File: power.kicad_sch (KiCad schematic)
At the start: 40 parts, among them SW7 Switch, U11 SY8079AAC, U12 SY8079AAC, U13 XT4054K421MR-G, U14 SY6280AAC, U15 SY6280AAC, U16 SY6280AAC

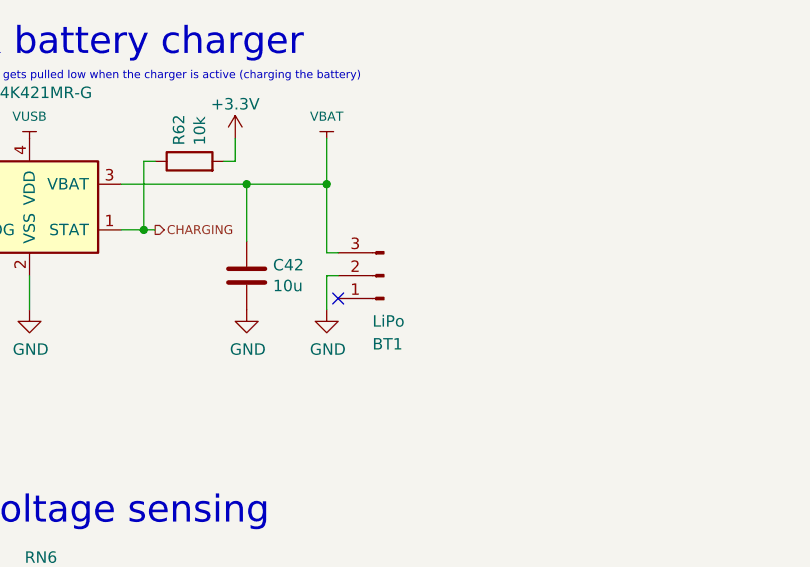
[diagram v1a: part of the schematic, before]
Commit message: Final version of prototype 4
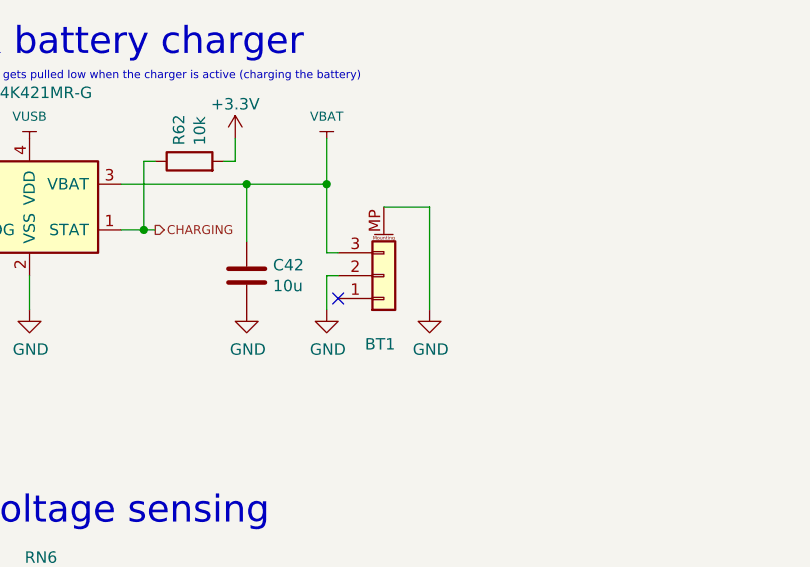
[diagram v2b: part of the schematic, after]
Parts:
- BT1: value LiPo -> (none); footprint Connector_JST:JST_PH_S3B-PH-SM4-TB_1x03-1MP_P2.00mm_Horizontal -> (none); symbol mch2021-rescue:Conn_01x03_Male-Connector -> Connector_Generic_MountingPin:Conn_01x03_MountingPin
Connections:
- net GND: now also BT1.MP (MountPin)
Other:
- moved on the sheet: BT1
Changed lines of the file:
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@@
+    (stroke (width 0) (type default) (color 0 0 0 0))
+  )
+  (wire (pts (xy 96.52 34.29) (xy 91.44 34.29))
     (stroke (width 0) (type default) (color 0 0 0 0))
   )
@@
   )
   (wire (pts (xy 58.42 85.09) (xy 64.77 85.09))
+    (stroke (width 0) (type default) (color 0 0 0 0))
+  )
+  (wire (pts (xy 96.52 45.72) (xy 96.52 34.29))
     (stroke (width 0) (type default) (color 0 0 0 0))
   )
@@
     (pin "1")
   )
-  (symbol (lib_id "mch2021-rescue:Conn_01x03_Male-Connector") (at 91.44 41.91 180) (unit 1)
-    (in_bom yes) (on_board yes)
-    (property "Reference" "BT1" (id 0) (at 90.17 49.53 0)
+  (symbol (lib_id "Connector_Generic_MountingPin:Conn_01x03_MountingPin") (at 91.44 41.91 0) (mirror x) (unit 1)
+    (in_bom yes) (on_board yes)
+    (property "Reference" "BT1" (id 0) (at 92.71 49.53 0)
       (effects (font (size 1.27 1.27)) (justify right))
     )
-    (property "Value" "LiPo" (id 1) (at 90.17 46.99 0)
+    (property "Value" "" (id 1) (at 92.71 46.99 0)
       (effects (font (size 1.27 1.27)) (justify right))
     )
-    (property "Footprint" "Connector_JST:JST_PH_S3B-PH-SM4-TB_1x03-1MP_P2.00mm_Horizontal" (id 2) (at 91.44 41.91 0)
+    (property "Footprint" "" (id 2) (at 91.44 41.91 0)
       (effects (font (size 1.27 1.27)) hide)
     )
@@
     (pin "2")
     (pin "3")
+    (pin "MP")
   )
   (symbol (lib_id "mch2021-rescue:AAT4610BIGV-1-T1-Power_Management") (at 156.21 109.22 0) (unit 1)
@@
     (pin "2")
   )
+  (symbol (lib_id "mch2021-rescue:GND-power") (at 96.52 45.72 0) (unit 1)
+    (in_bom yes) (on_board yes)
+    (property "Reference" "#PWR?" (id 0) (at 96.52 52.07 0)
+      (effects (font (size 1.27 1.27)) hide)
+    )
+    (property "Value" "GND" (id 1) (at 96.647 50.1142 0))
+    (property "Footprint" "" (id 2) (at 96.52 45.72 0)
+      (effects (font (size 1.27 1.27)) hide)
+    )
+    (property "Datasheet" "" (id 3) (at 96.52 45.72 0)
+      (effects (font (size 1.27 1.27)) hide)
+    )
+    (pin "1")
+  )
 )
